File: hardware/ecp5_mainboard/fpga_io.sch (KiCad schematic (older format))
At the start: 75 parts, among them J10 UART, J11 FLASH, J12 JTAG, J5 EXT0, J6 EXT1, J7 EXT2, J8 EXT3, J9 PMOD_01, Q9 BSH111BKR, SW6 SW_Push, U15 ECP5UM5G_85_CABGA756, U26 XL_XO_LVDS, U27 W25Q

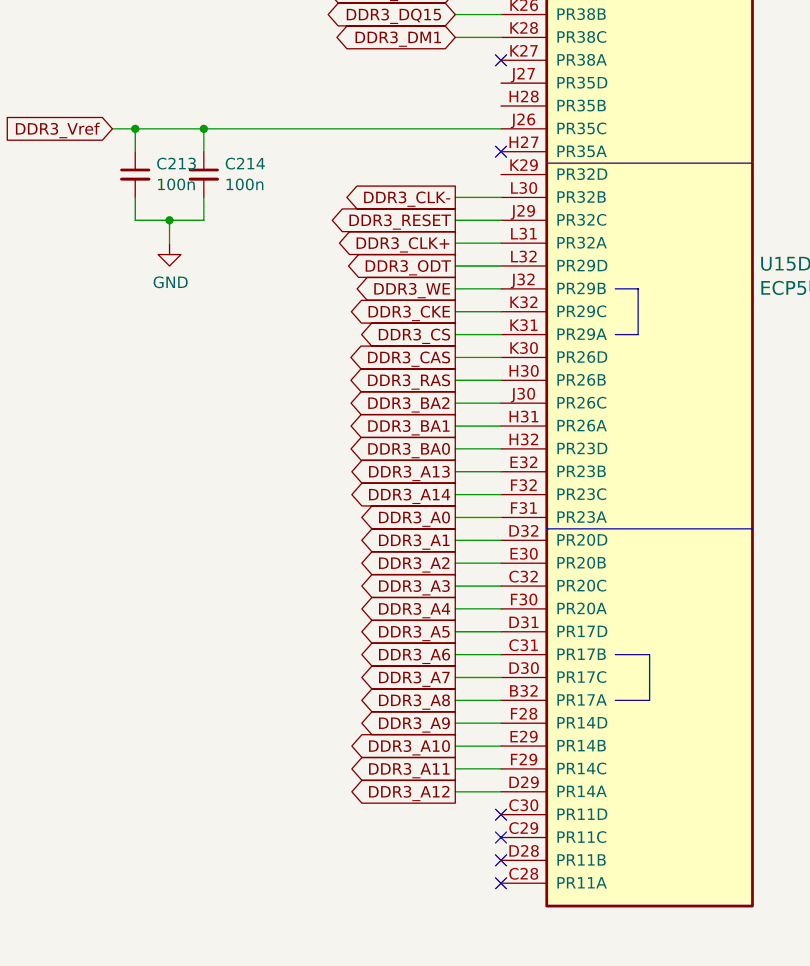
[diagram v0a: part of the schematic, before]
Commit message: hardware/mainboard: DDR3 Address routing
Signed-off-by: David Shah <dave@ds0.me>
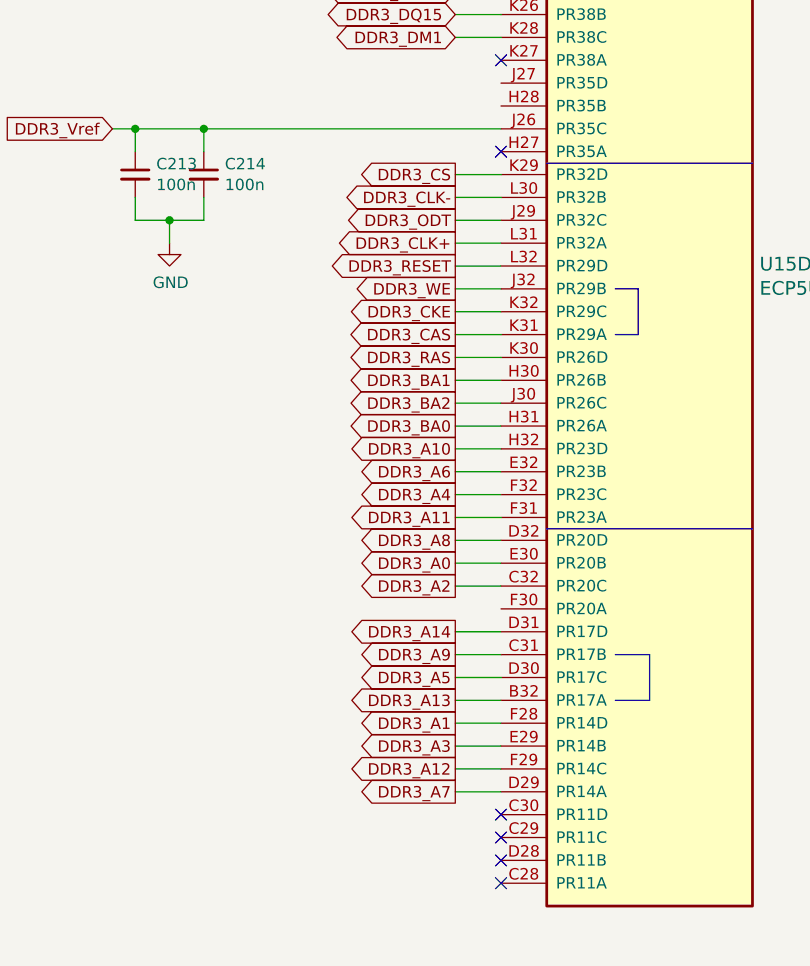
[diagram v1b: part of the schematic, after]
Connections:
- net DDR3_A0: now also U15.E30 (PR20B); no longer U15.F31 (PR23A)
- net DDR3_A1: now also U15.F28 (PR14D); no longer U15.D32 (PR20D)
- net DDR3_A10: now also U15.H32 (PR23D); no longer U15.E29 (PR14B)
- net DDR3_A11: now also U15.F31 (PR23A); no longer U15.F29 (PR14C)
- net DDR3_A12: now also U15.F29 (PR14C); no longer U15.D29 (PR14A)
- net DDR3_A13: now also U15.B32 (PR17A); no longer U15.E32 (PR23B)
- net DDR3_A14: now also U15.D31 (PR17D); no longer U15.F32 (PR23C)
- net DDR3_A2: now also U15.C32 (PR20C); no longer U15.E30 (PR20B)
- net DDR3_A3: now also U15.E29 (PR14B); no longer U15.C32 (PR20C)
- net DDR3_A4: now also U15.F32 (PR23C); no longer U15.F30 (PR20A)
- net DDR3_A5: now also U15.D30 (PR17C); no longer U15.D31 (PR17D)
- net DDR3_A6: now also U15.E32 (PR23B); no longer U15.C31 (PR17B)
- net DDR3_A7: now also U15.D29 (PR14A); no longer U15.D30 (PR17C)
- net DDR3_A8: now also U15.D32 (PR20D); no longer U15.B32 (PR17A)
- net DDR3_A9: now also U15.C31 (PR17B); no longer U15.F28 (PR14D)
- net DDR3_BA0: now also U15.H31 (PR26A); no longer U15.H32 (PR23D)
- net DDR3_BA1: now also U15.H30 (PR26B); no longer U15.H31 (PR26A)
- net DDR3_CAS: now also U15.K31 (PR29A); no longer U15.K30 (PR26D)
- net DDR3_CS: now also U15.K29 (PR32D); no longer U15.K31 (PR29A)
- net DDR3_ODT: now also U15.J29 (PR32C); no longer U15.L32 (PR29D)
- net DDR3_RAS: now also U15.K30 (PR26D); no longer U15.H30 (PR26B)
- net DDR3_RESET: now also U15.L32 (PR29D); no longer U15.J29 (PR32C)
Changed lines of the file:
@@
 Wire Wire Line
 	5400 4300 5600 4300
+Text GLabel 2150 5250 0    50   Output ~ 0
+DDR3_A0
+Text GLabel 2150 5950 0    50   Output ~ 0
+DDR3_A1
+Text GLabel 2150 5350 0    50   Output ~ 0
+DDR3_A2
+Text GLabel 2150 6050 0    50   Output ~ 0
+DDR3_A3
+Text GLabel 2150 4950 0    50   Output ~ 0
+DDR3_A4
+Text GLabel 2150 5750 0    50   Output ~ 0
+DDR3_A5
+Text GLabel 2150 4850 0    50   Output ~ 0
+DDR3_A6
+Text GLabel 2150 6250 0    50   Output ~ 0
+DDR3_A7
+Text GLabel 2150 5150 0    50   Output ~ 0
+DDR3_A8
+Text GLabel 2150 5650 0    50   Output ~ 0
+DDR3_A9
+Text GLabel 2150 4750 0    50   Output ~ 0
+DDR3_A10
 Text GLabel 2150 5050 0    50   Output ~ 0
-DDR3_A0
-Text GLabel 2150 5150 0    50   Output ~ 0
-DDR3_A1
-Text GLabel 2150 5250 0    50   Output ~ 0
-DDR3_A2
-Text GLabel 2150 5350 0    50   Output ~ 0
-DDR3_A3
-Text GLabel 2150 5450 0    50   Output ~ 0
-DDR3_A4
+DDR3_A11
+Text GLabel 2150 6150 0    50   Output ~ 0
+DDR3_A12
+Text GLabel 2150 5850 0    50   Output ~ 0
+DDR3_A13
 Text GLabel 2150 5550 0    50   Output ~ 0
-DDR3_A5
-Text GLabel 2150 5650 0    50   Output ~ 0
-DDR3_A6
-Text GLabel 2150 5750 0    50   Output ~ 0
-DDR3_A7
-Text GLabel 2150 5850 0    50   Output ~ 0
-DDR3_A8
-Text GLabel 2150 5950 0    50   Output ~ 0
-DDR3_A9
-Text GLabel 2150 6050 0    50   Output ~ 0
-DDR3_A10
-Text GLabel 2150 6150 0    50   Output ~ 0
-DDR3_A11
-Text GLabel 2150 6250 0    50   Output ~ 0
-DDR3_A12
-Text GLabel 2150 4850 0    50   Output ~ 0
-DDR3_A13
-Text GLabel 2150 4950 0    50   Output ~ 0
 DDR3_A14
+Wire Wire Line
+	2150 5250 2350 5250
+Wire Wire Line
+	2150 5950 2350 5950
+Wire Wire Line
+	2150 5350 2350 5350
+Wire Wire Line
+	2150 6050 2350 6050
+Wire Wire Line
+	2150 4950 2350 4950
+Wire Wire Line
+	2150 5750 2350 5750
+Wire Wire Line
+	2150 4850 2350 4850
+Wire Wire Line
+	2150 6250 2350 6250
+Wire Wire Line
+	2150 5150 2350 5150
+Wire Wire Line
+	2150 5650 2350 5650
+Wire Wire Line
+	2150 4750 2350 4750
 Wire Wire Line
 	2150 5050 2350 5050
 Wire Wire Line
-	2150 5150 2350 5150
-Wire Wire Line
-	2150 5250 2350 5250
-Wire Wire Line
-	2150 5350 2350 5350
-Wire Wire Line
-	2150 5450 2350 5450
-Wire Wire Line
-	2150 5550 2350 5550
-Wire Wire Line
-	2150 5650 2350 5650
-Wire Wire Line
-	2150 5750 2350 5750
+	2150 6150 2350 6150
 Wire Wire Line
 	2150 5850 2350 5850
 Wire Wire Line
-	2150 5950 2350 5950
-Wire Wire Line
-	2150 6050 2350 6050
-Wire Wire Line
-	2150 6150 2350 6150
-Wire Wire Line
-	2150 6250 2350 6250
-Wire Wire Line
-	2150 4850 2350 4850
-Wire Wire Line
-	2150 4950 2350 4950
+	2150 5550 2350 5550
 NoConn ~ 5600 6600
-Text GLabel 2150 4750 0    50   Output ~ 0
+Text GLabel 2150 4650 0    50   Output ~ 0
 DDR3_BA0
-Text GLabel 2150 4650 0    50   Output ~ 0
+Text GLabel 2150 4450 0    50   Output ~ 0
 DDR3_BA1
 Text GLabel 2150 4550 0    50   Output ~ 0
 DDR3_BA2
-Text GLabel 2150 4450 0    50   Output ~ 0
+Text GLabel 2150 4350 0    50   Output ~ 0
 DDR3_RAS
-Text GLabel 2150 4350 0    50   Output ~ 0
+Text GLabel 2150 4250 0    50   Output ~ 0
 DDR3_CAS
 Text GLabel 2150 4150 0    50   Output ~ 0
@@
 Text GLabel 2150 4050 0    50   Output ~ 0
 DDR3_WE
+Text GLabel 2150 3750 0    50   Output ~ 0
+DDR3_ODT
 Text GLabel 2150 3950 0    50   Output ~ 0
-DDR3_ODT
-Text GLabel 2150 3750 0    50   Output ~ 0
 DDR3_RESET
-Text GLabel 2150 4250 0    50   Output ~ 0
+Text GLabel 2150 3550 0    50   Output ~ 0
 DDR3_CS
 Text GLabel 5400 5000 0    50   BiDi ~ 0
@@
 	5400 5000 5600 5000
 Wire Wire Line
+	2150 3950 2350 3950
+Wire Wire Line
 	2150 3750 2350 3750
-Wire Wire Line
-	2150 3950 2350 3950
 Wire Wire Line
 	2150 4050 2350 4050
@@
 	2150 4150 2350 4150
 Wire Wire Line
+	2150 3550 2350 3550
+Wire Wire Line
 	2150 4250 2350 4250
 Wire Wire Line
 	2150 4350 2350 4350
 Wire Wire Line
+	2150 4550 2350 4550
+Wire Wire Line
 	2150 4450 2350 4450
 Wire Wire Line
-	2150 4550 2350 4550
-Wire Wire Line
 	2150 4650 2350 4650
-Wire Wire Line
-	2150 4750 2350 4750
 Text GLabel 2150 3850 0    50   Output ~ 0
 DDR3_CLK+
